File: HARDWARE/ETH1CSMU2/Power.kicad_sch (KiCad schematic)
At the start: 43 parts, among them Q801 IRFR5410, U801 TMR 4-2411WI, U802 TEL 12-2423, U803 NCV1117DT33T5G, U804 MAX5902

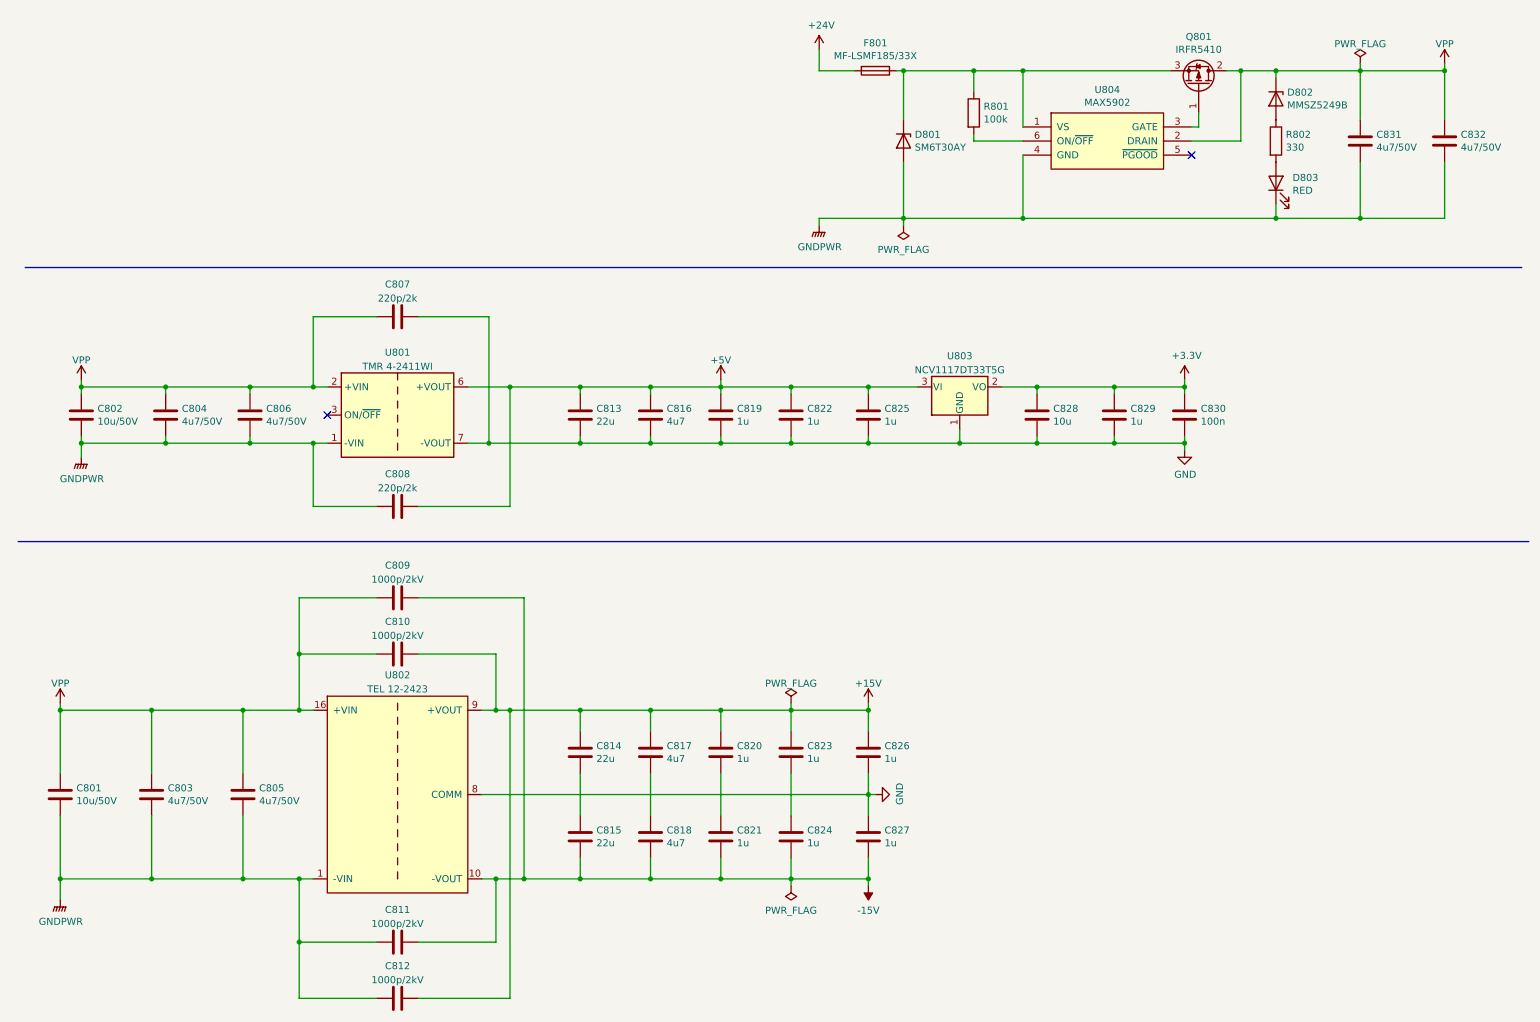
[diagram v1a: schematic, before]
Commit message: Hardware design
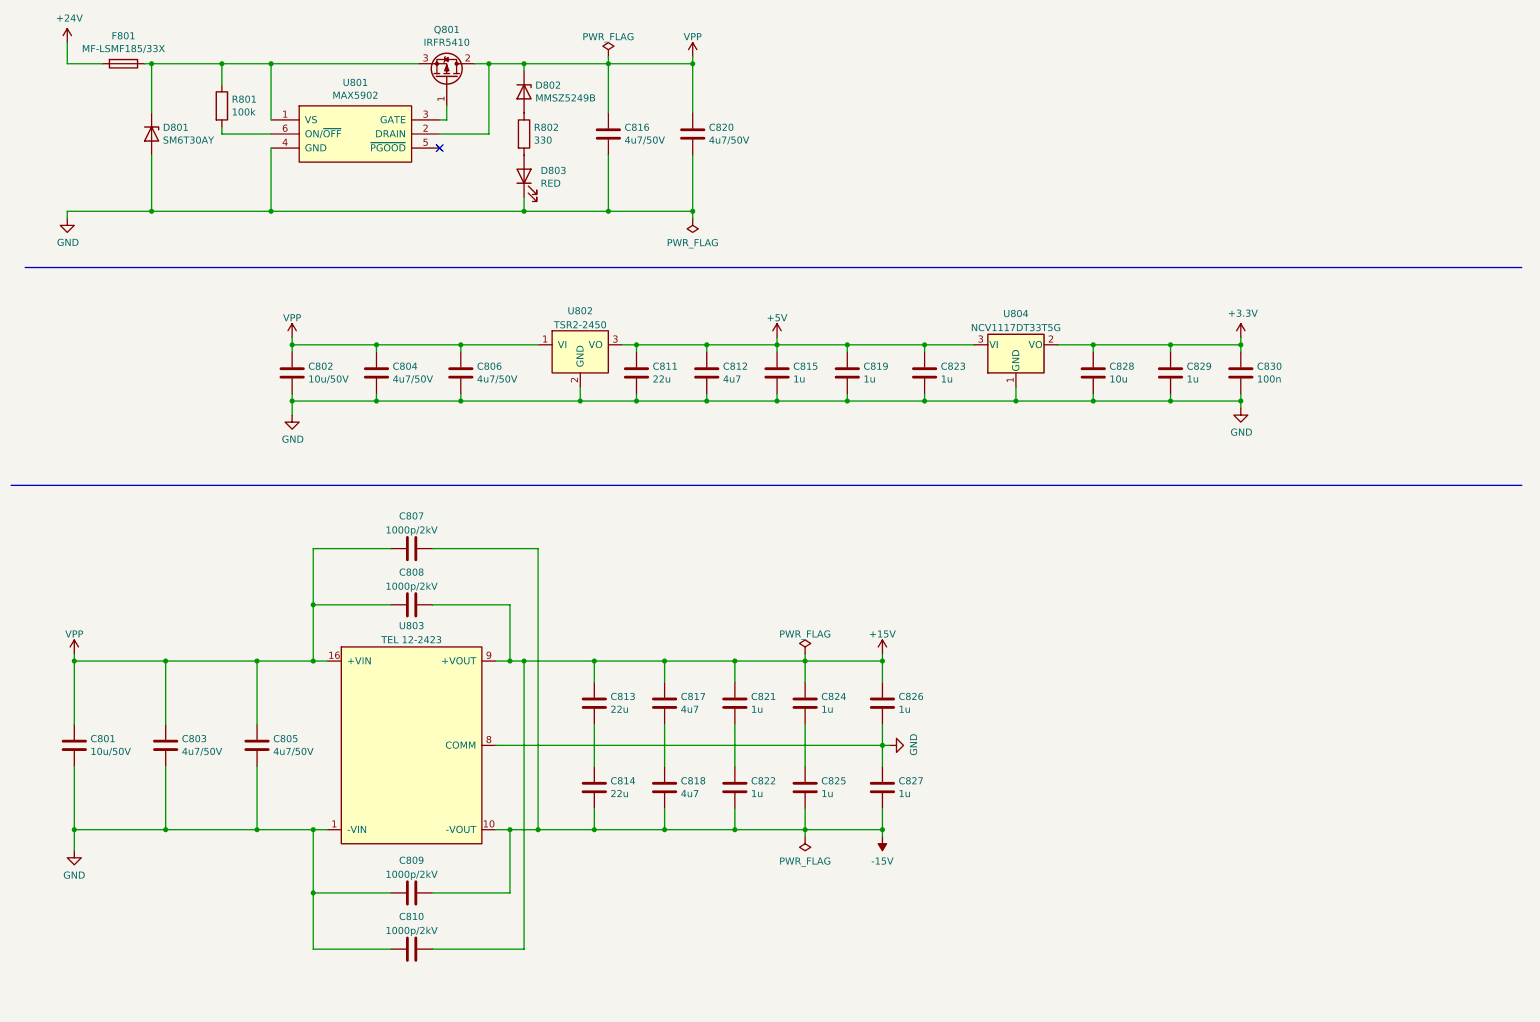
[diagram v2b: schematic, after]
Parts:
- removed C807, C808: 220p/2k, Capacitor_SMD:C_1812_4532Metric_Pad1.57x3.40mm_HandSolder, symbol Device:C
- removed U801: TMR 4-2411WI, ETH1CSMU2:TRM 4-SINGLE, symbol Converter_DCDC:TMR-2411
- added U802: TSR2-2450, ETH1CSMU2:TSR2, symbol ETH1CSMU2:TSR2
- renumbered C809 to C807, C810 to C808, C811 to C809, C812 to C810, C813 to C811, C816 to C812, C814 to C813, C815 to C814, C819 to C815, C831 to C816, C822 to C819, C832 to C820, C820 to C821, C821 to C822, C825 to C823, C823 to C824, C824 to C825, U804 to U801, U802 to U803, U803 to U804
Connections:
- net GNDPWR is gone; now on net GND: C801.2, C802.2, C803.2, C804.2, C805.2, C806.2, C809.1, C810.1, C816.2, C820.2, D801.2 (A), D803.1 (K), U801.4 (GND), U803.1 (-VIN)
- net +5V: now also U802.3 (VO)
- net GND: now also U802.2 (GND)
- net VPP: now also U802.1 (VI)
- no-connect marks 2 -> 1
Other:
- moved on the sheet: C801, C802, C803, C804, C805, C806, C807, C808, C809, C810, C811, C812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
